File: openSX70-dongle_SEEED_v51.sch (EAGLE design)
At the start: 24 parts, among them SW1 MK-12C02 G1.5, SW2 MK-12C02 G1.5, X1 1503_02

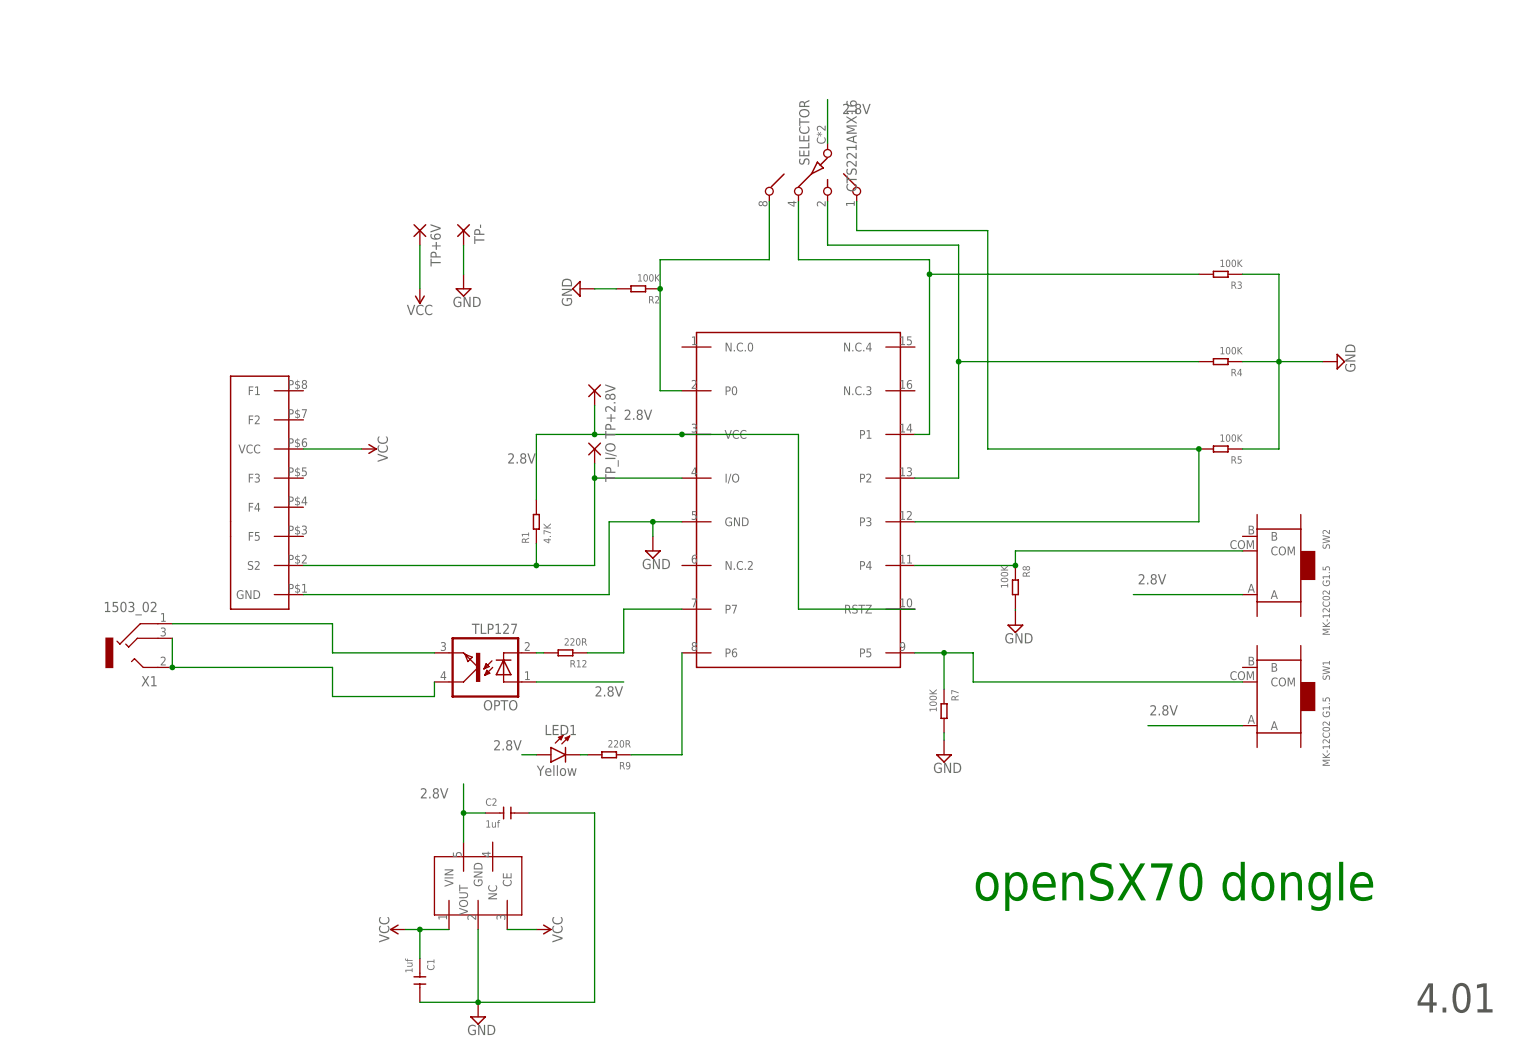
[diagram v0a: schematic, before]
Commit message: no message
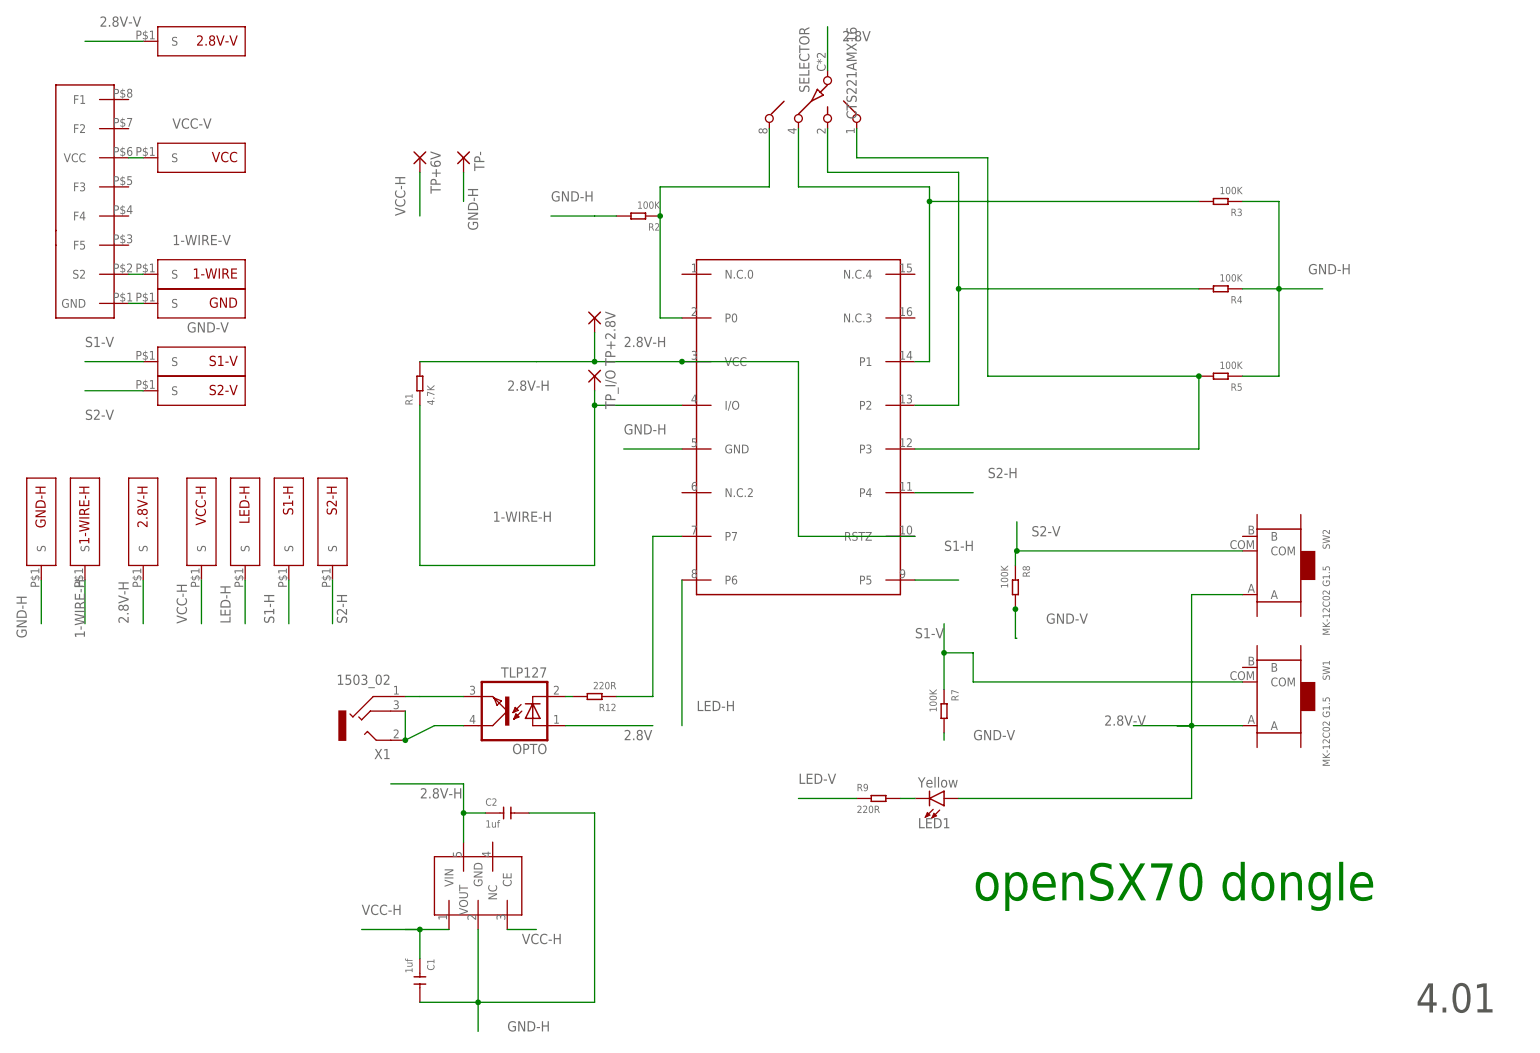
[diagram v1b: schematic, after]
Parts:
- added 1-WIRE, 1-WIRE-H, 2.8V-H, 2.8V-V, GND, GND-H, LED-H, S1-H, S1-V, S2-H, S2-V, VCC, VCC-H: SX70-S-PAD-NEW, openSX70:SX70-S-PAD-NEW
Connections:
- removed net GND: C1.2, C2.2, DS2408.GND, R2.2, R3.1, R4.1, R5.1, R7.2, R8.2, REG.GND, TP-.P, U$1.GND
- removed net N$1: DS2408.I/O, R1.1, TP_I/O.P, U$1.S2
- removed net N$6: DS2408.P4, R8.1, SW2.COM
- removed net N$7: DS2408.P5, R7.1, SW1.COM
- removed net N$8: DS2408.P6, R9.1
- removed net VCC: C1.1, REG.CE, REG.VIN, TP+6V.P, U$1.VCC
- new net 1-WIRE-H: 1-WIRE-H.S, DS2408.I/O, R1.1, TP_I/O.P
- new net 1-WIRE-V: 1-WIRE.S, U$1.S2
- new net 2.8V-H: 2.8V-H.S, C2.1, DS2408.RSTZ, DS2408.VCC, R1.2, REG.VOUT, TP+2.8V.P
- new net 2.8V-V: 2.8V-V.S, LED1.A, SW1.A, SW2.A
- new net GND-H: C1.2, C2.2, DS2408.GND, GND-H.S, R2.2, R3.1, R4.1, R5.1, REG.GND, TP-.P
- new net GND-V: GND.S, R7.2, R8.2, U$1.GND
- new net LED-H: DS2408.P6, LED-H.S
- new net LED-V: R9.1
- new net S1-H: DS2408.P5, S1-H.S
- new net S1-V: R7.1, S1-V.S, SW1.COM
- new net S2-H: DS2408.P4, S2-H.S
- new net S2-V: R8.1, S2-V.S, SW2.COM
- new net VCC-H: C1.1, REG.CE, REG.VIN, TP+6V.P, VCC-H.S
- new net VCC-V: U$1.VCC, VCC.S
- net 2.8V: no longer C2.1, DS2408.RSTZ, DS2408.VCC, LED1.A, R1.2, REG.VOUT, SW1.A, SW2.A, TP+2.8V.P
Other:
- moved on the sheet: LED1, OPTO, R1, R12, R2, R3, R4, R5, R9, SELECTOR, TP+2.8V, TP+6V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
